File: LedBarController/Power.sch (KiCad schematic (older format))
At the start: 25 parts, among them J1201 Barrel_Jack_Switch, Q1201 FQP47P06, U1201 AMS1117-5.0, U1202 INA219AxD

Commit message: Route complete
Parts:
- D1203: Price (none) -> 0.1; is stock (none) -> no
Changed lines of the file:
@@
 F 2 "Diode_SMD:D_SMB_Handsoldering" H 3000 3750 50  0001 C CNN
 F 3 "~" H 3000 3750 50  0001 C CNN
+F 4 "0.1" H 3000 3750 50  0001 C CNN "Price"
+F 5 "no" H 3000 3750 50  0001 C CNN "is stock"
 	1    3000 3750
 	0    1    1    0

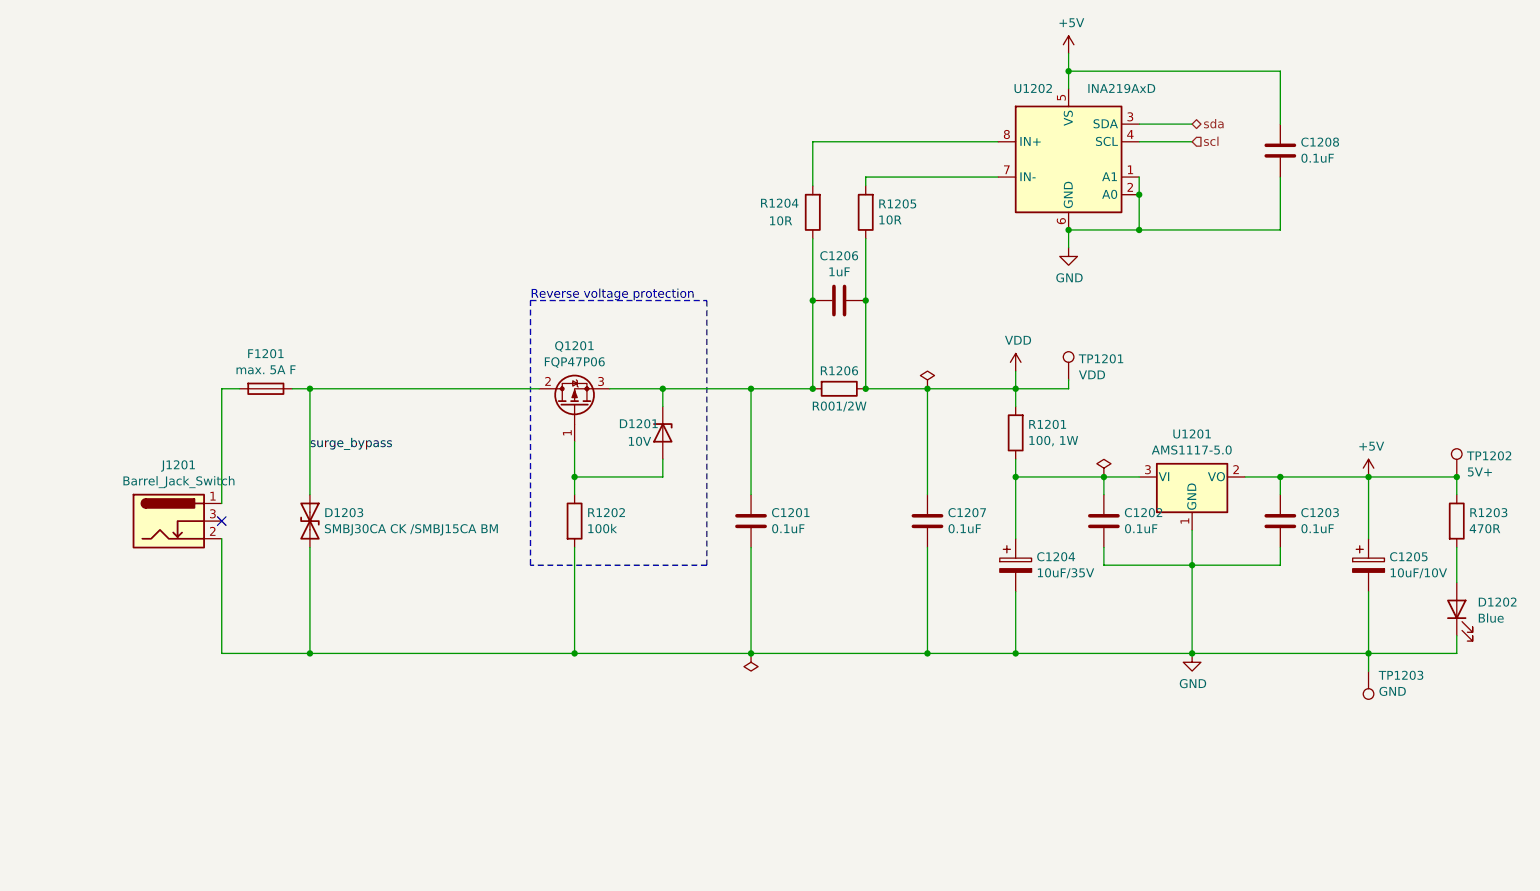
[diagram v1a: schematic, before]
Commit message: moved board on schema to same sheet
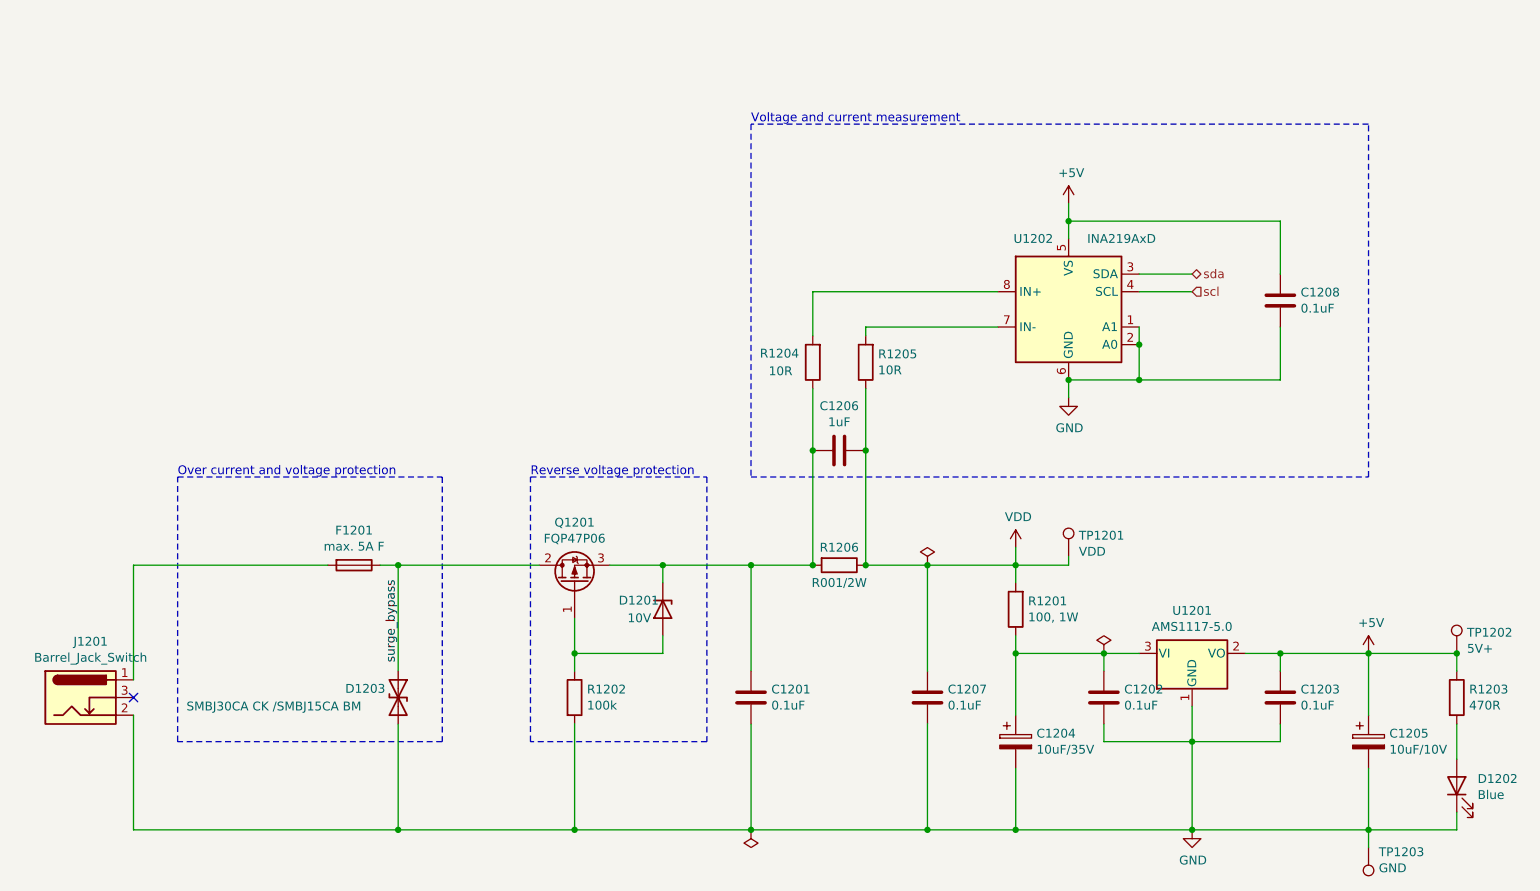
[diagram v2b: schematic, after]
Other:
- note added: "Over current and voltage protection"
- note added: "Voltage and current measurement"
- moved on the sheet: C1201, C1202, C1203, C1204, C1205, C1206, C1207, C1208, D1201, D1202, D1203, F1201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
